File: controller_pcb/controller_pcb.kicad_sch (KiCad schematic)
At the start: 4 parts, among them IC1 ATTINY85V-10SU

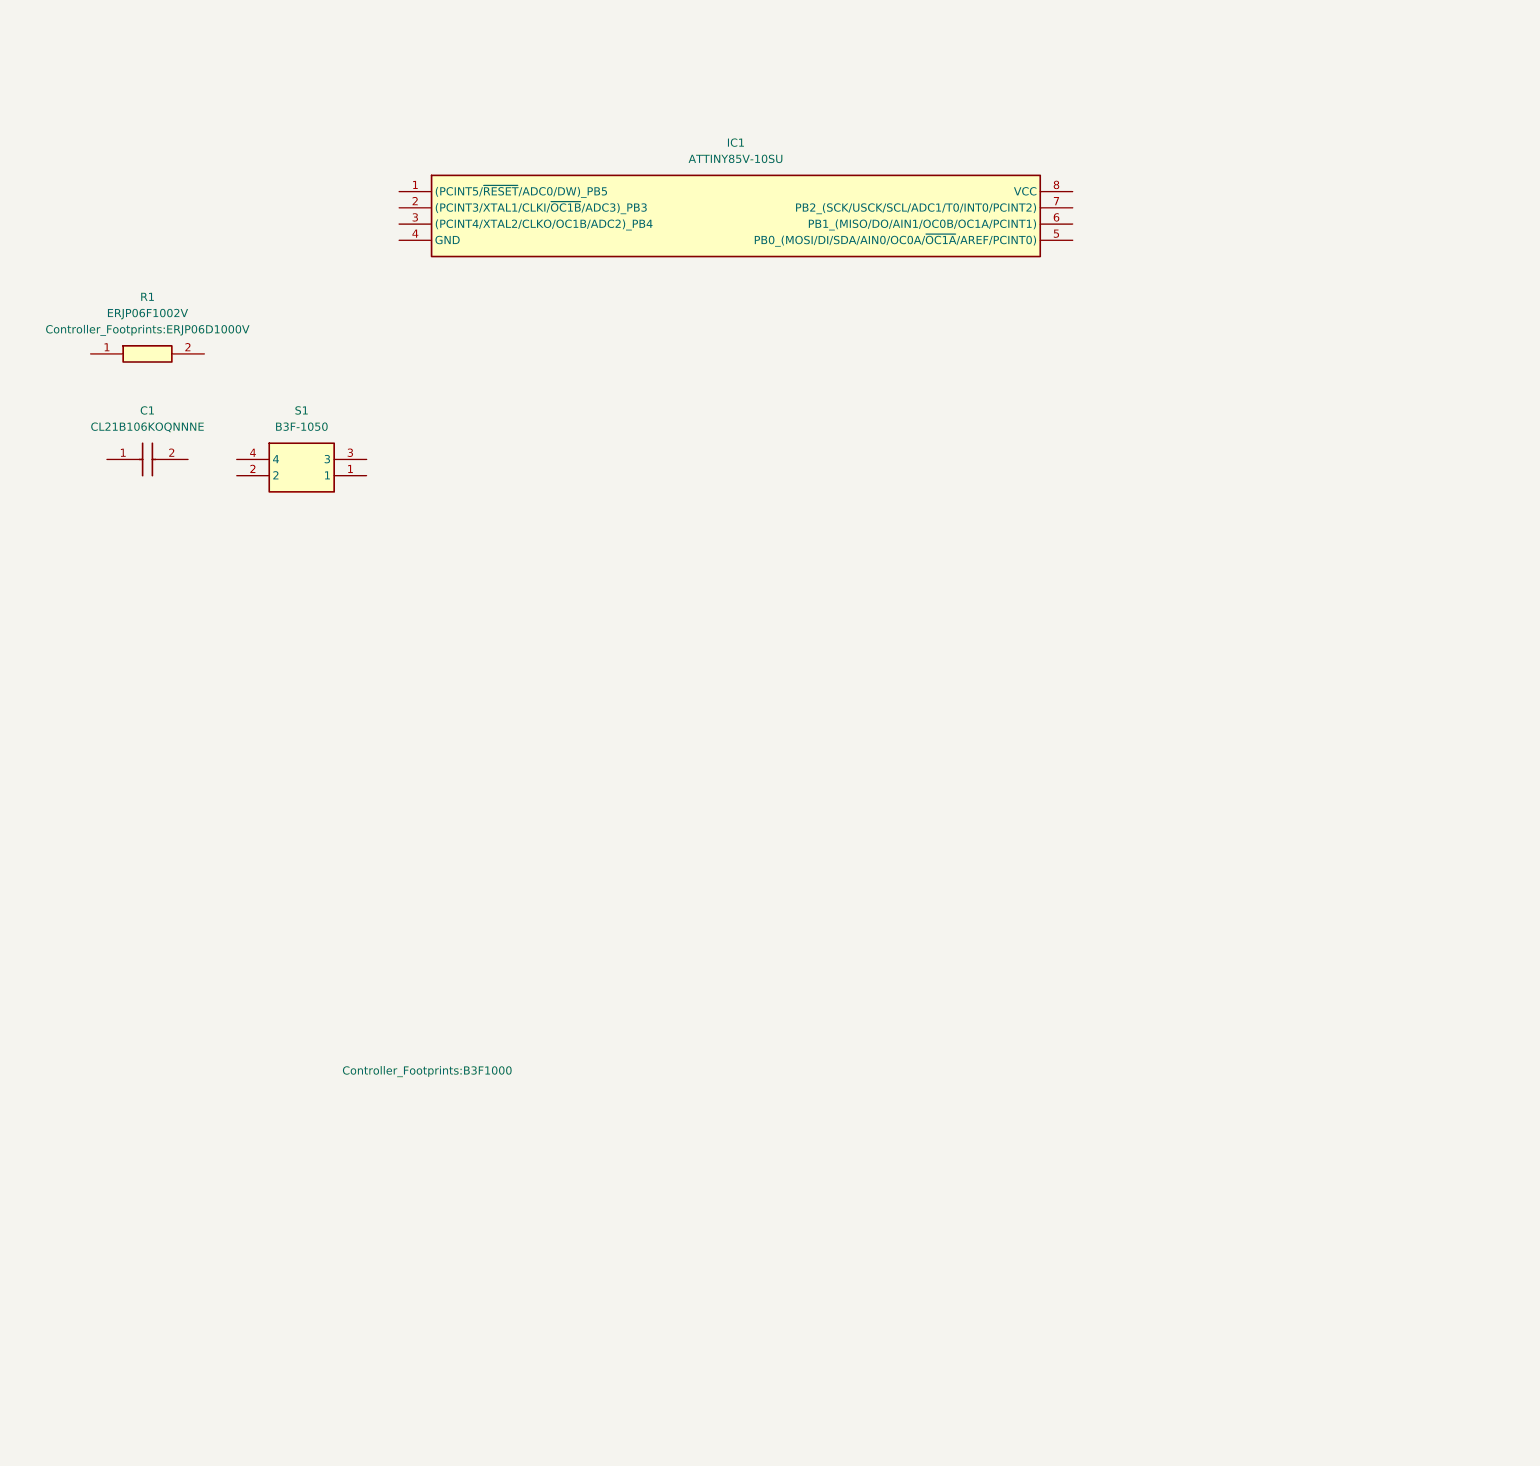
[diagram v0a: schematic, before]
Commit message: Started placing and wiring
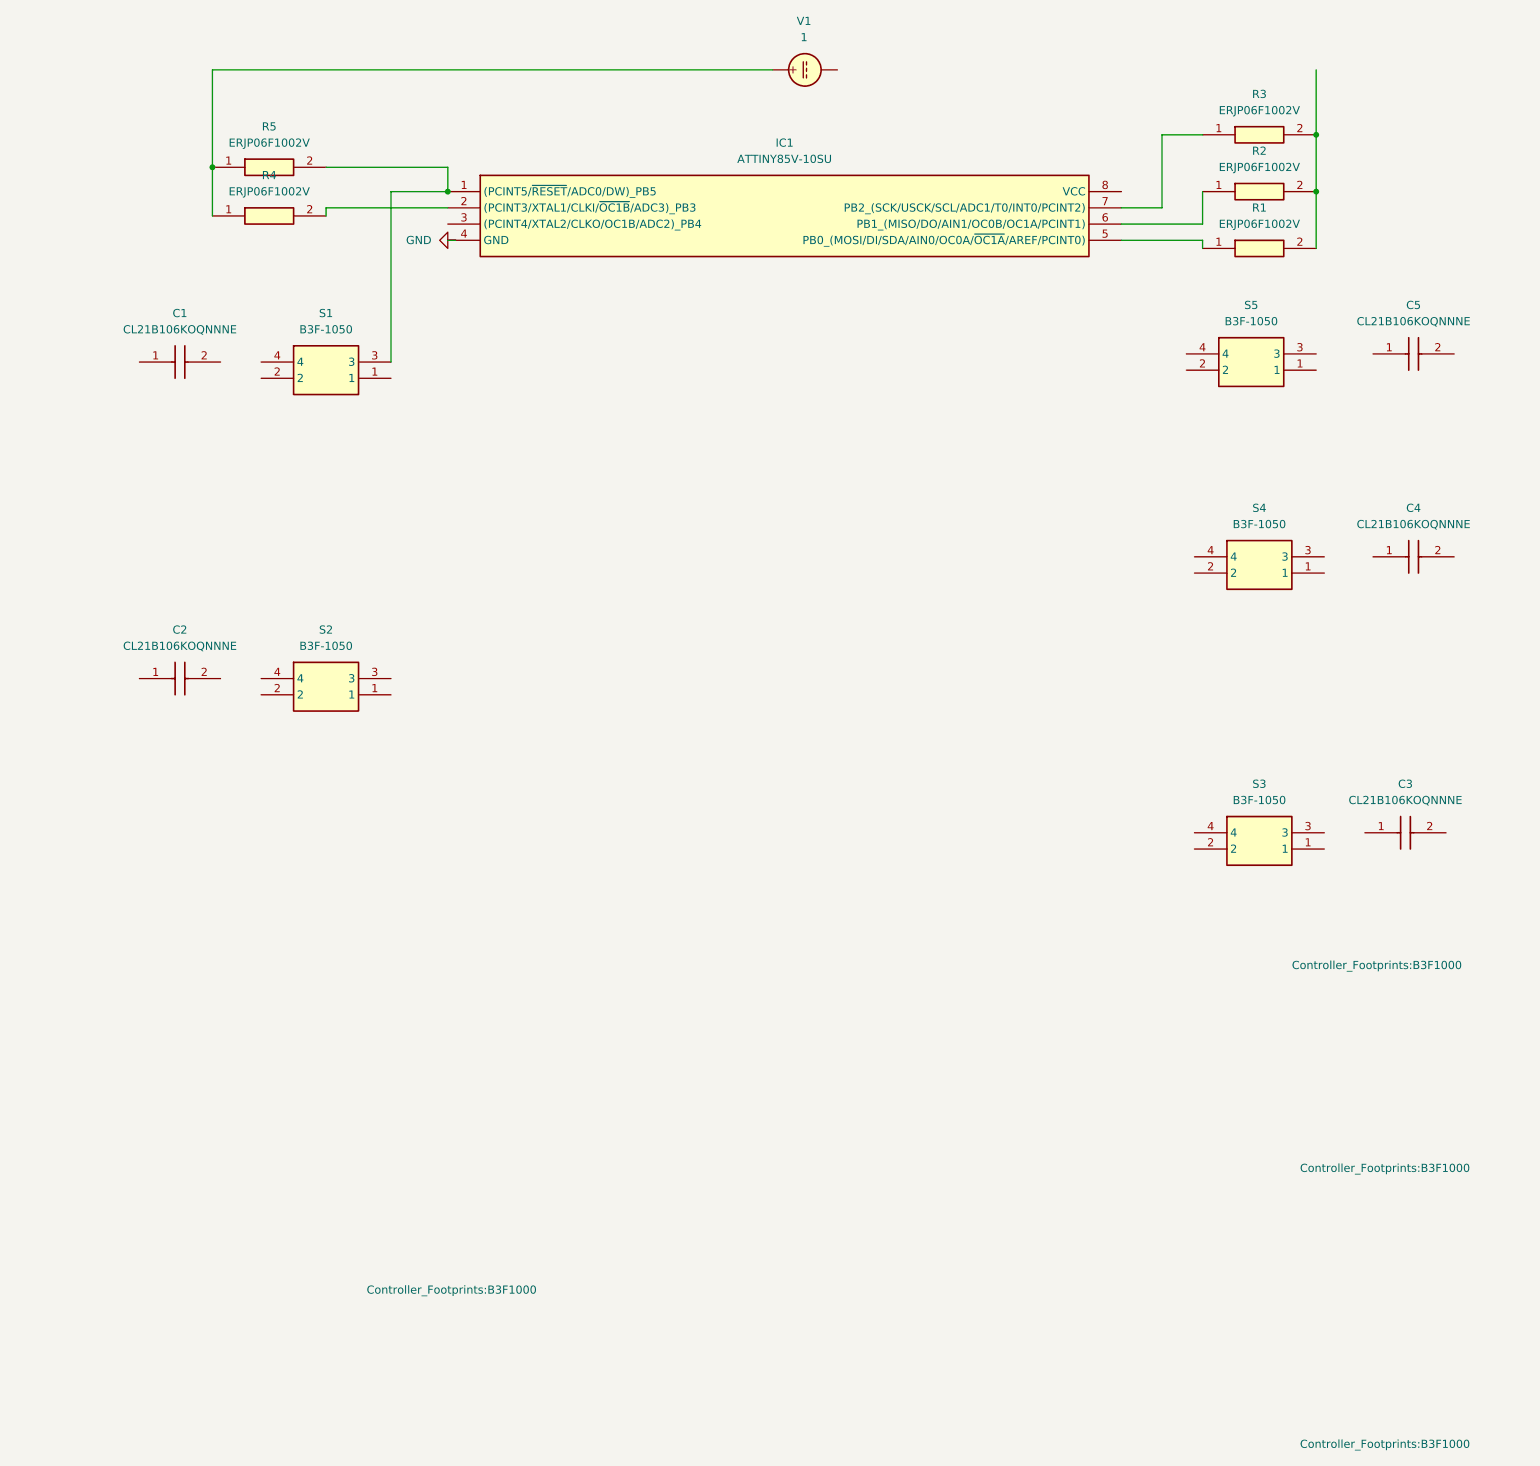
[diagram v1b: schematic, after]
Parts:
- added C2, C3, C4, C5: CL21B106KOQNNNE, CAPC2012X140N, symbol Controller_Comp:CL21B106KOQNNNE
- added R2, R3, R4, R5: ERJP06F1002V, Controller_Footprints:ERJP06D1000V, symbol Controller_Comp:ERJP06F1002V
- added S2, S3, S4, S5: B3F-1050, Controller_Footprints:B3F1000, symbol Controller_Comp:B3F-1050
- added V1: 1, symbol Simulation_SPICE:VDC
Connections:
- net at IC1.1 ((PCINT5/~{RESET}/ADC0/DW)_PB5): now also S1.3, R5.2
- net at IC1.2 ((PCINT3/XTAL1/CLKI/~{OC1B}/ADC3)_PB3): now also R4.2
- net GND: now reaches IC1.4 (GND)
- net at IC1.5 (PB0_(MOSI/DI/SDA/AIN0/OC0A/~{OC1A}/AREF/PCINT0)): now also R1.1
- net at IC1.6 (PB1_(MISO/DO/AIN1/OC0B/OC1A/PCINT1)): now also R2.1
- net at IC1.7 (PB2_(SCK/USCK/SCL/ADC1/T0/INT0/PCINT2)): now also R3.1
- net at R1.2: now also R2.2, R3.2
- new net: R4.1, R5.1, V1.1
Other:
- moved on the sheet: C1, IC1, R1, S1

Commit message: Finished schematic, updating PCB
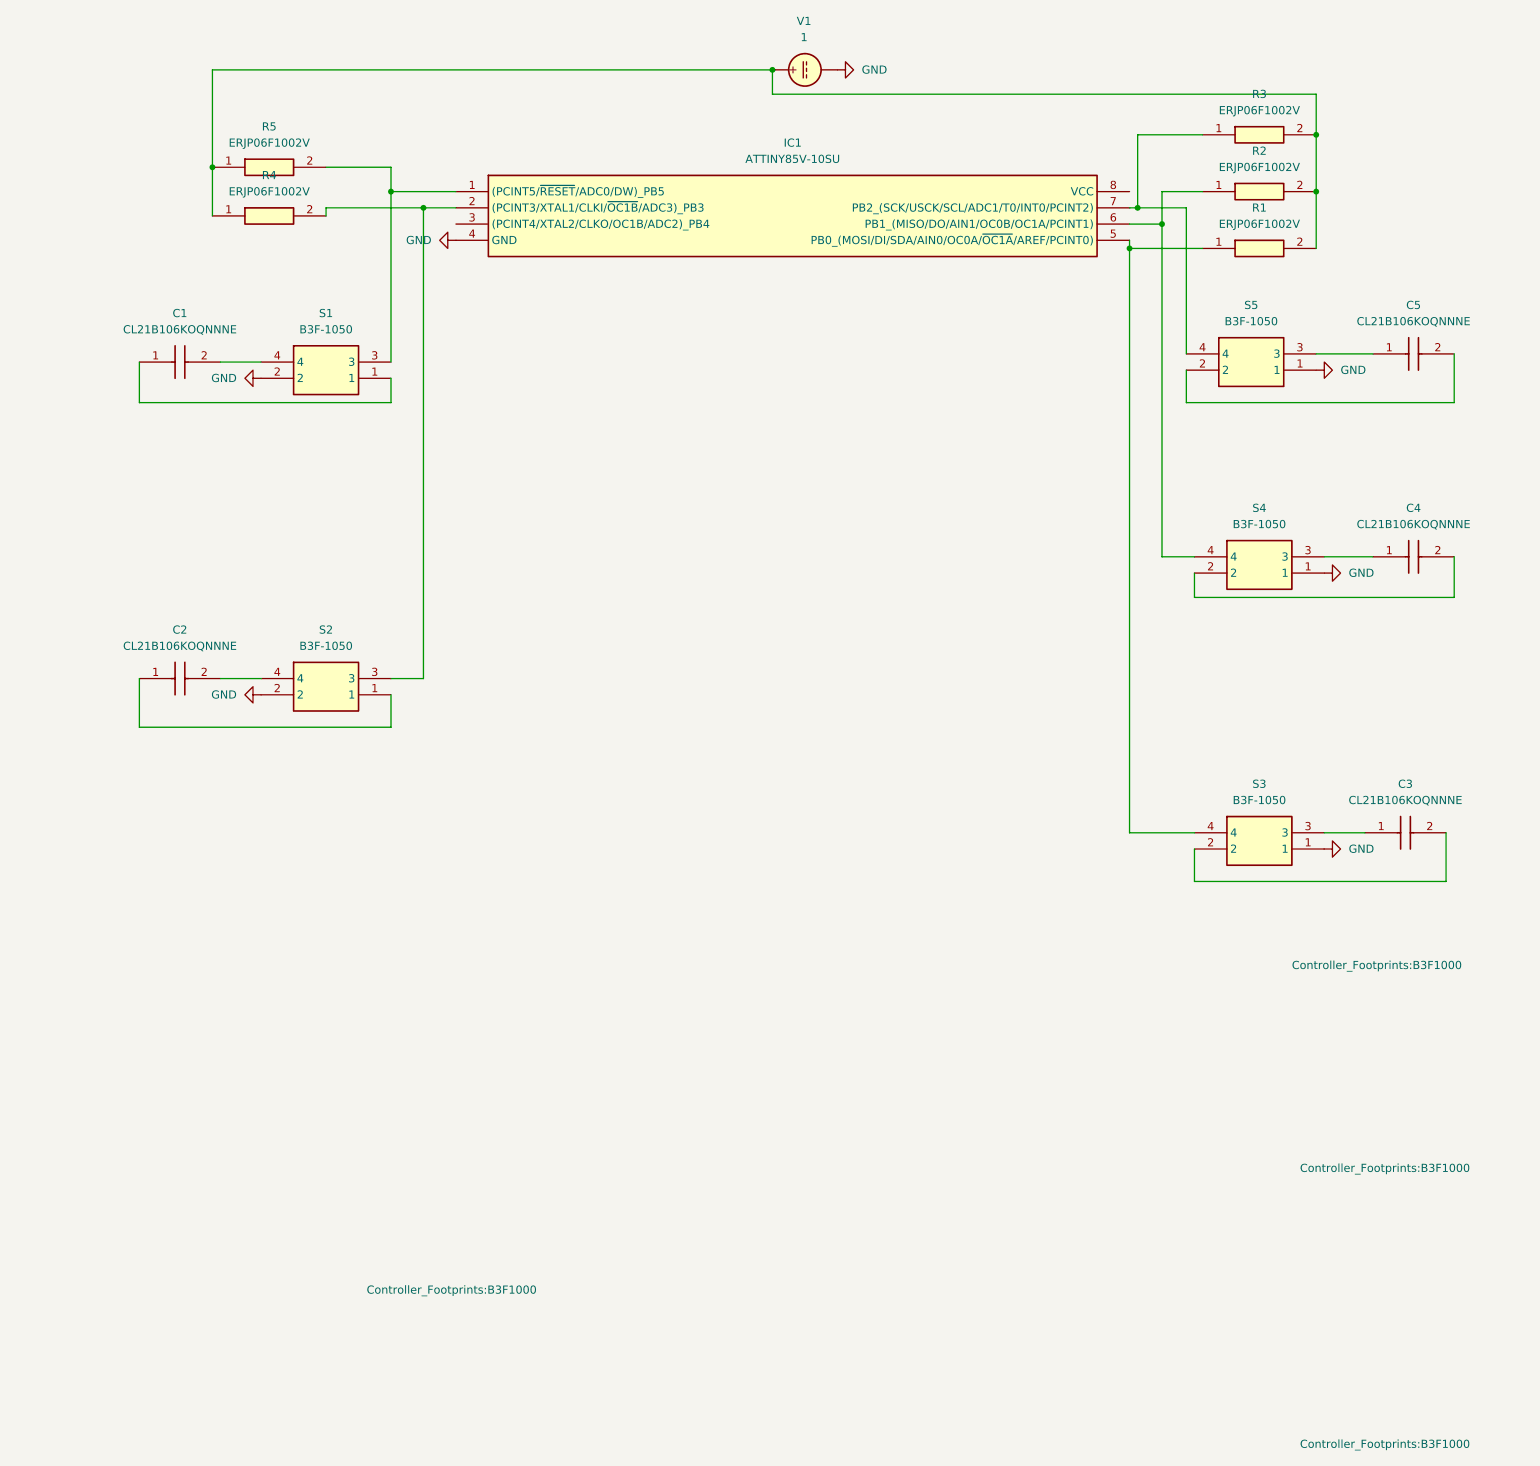
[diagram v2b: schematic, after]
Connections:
- net GND: now also S1.2, S2.2, S3.1, S4.1, S5.1, V1.2
- net at IC1.2 ((PCINT3/XTAL1/CLKI/~{OC1B}/ADC3)_PB3), R4.2: now also S2.3
- net at IC1.5 (PB0_(MOSI/DI/SDA/AIN0/OC0A/~{OC1A}/AREF/PCINT0)), R1.1: now also S3.4
- net at IC1.6 (PB1_(MISO/DO/AIN1/OC0B/OC1A/PCINT1)), R2.1: now also S4.4
- net at IC1.7 (PB2_(SCK/USCK/SCL/ADC1/T0/INT0/PCINT2)), R3.1: now also S5.4
- net at R4.1, R5.1, V1.1: now also R1.2, R2.2, R3.2
- net at C4.1: now also S4.3
- net at C4.2: now also S4.2
- net at C2.1: now also S2.1
- net at C2.2: now also S2.4
- net at C3.1: now also S3.3
- net at C3.2: now also S3.2
- net at C5.1: now also S5.3
- net at C5.2: now also S5.2
- net at S1.1: now also C1.1
- net at S1.4: now also C1.2
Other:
- moved on the sheet: IC1
